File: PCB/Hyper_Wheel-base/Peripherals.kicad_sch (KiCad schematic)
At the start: 18 parts, among them J1-1 Conn_01x06_Socket, J1-2 Conn_01x06_Pin, J2-1 Conn_01x04_Socket, U13 AS5600L-ASOM, U14 DRV5032FCDBZR, U3 AS5600L-ASOM, U8 DRV5032FCDBZR

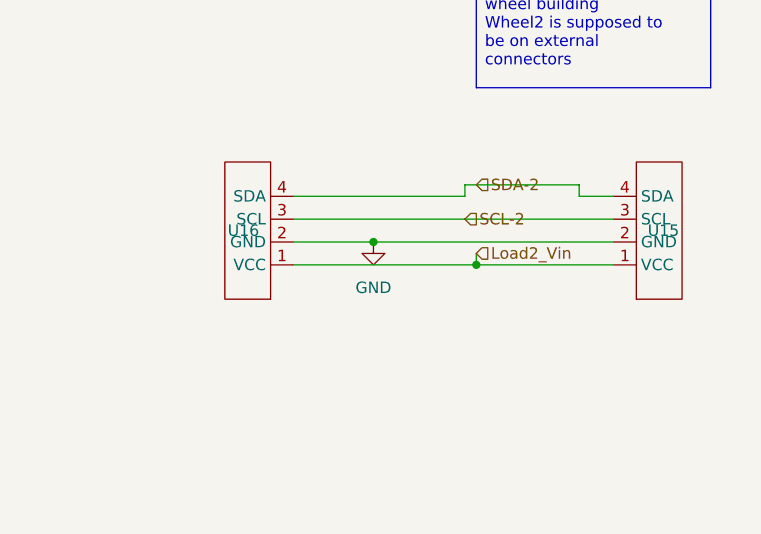
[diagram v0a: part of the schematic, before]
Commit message: Rev B Xiao.  migrated changes to main
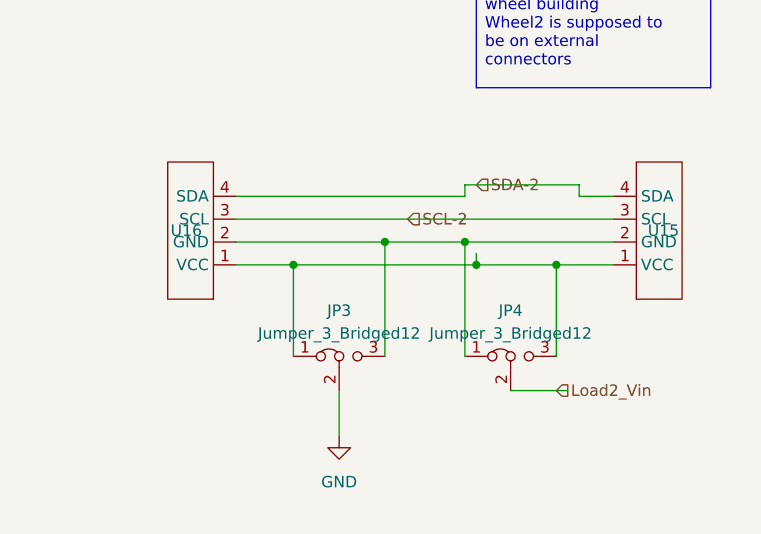
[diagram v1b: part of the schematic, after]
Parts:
- added JP3, JP4: Jumper_3_Bridged12, Jumper:SolderJumper-3_P1.3mm_Bridged12_Pad1.0x1.5mm, symbol Jumper:Jumper_3_Bridged12
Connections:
- net GND: now also JP3.2 (C); no longer U15.2 (GND), U16.2 (GND)
- net Load2_Vin: now also JP4.2 (C); no longer U15.1 (VCC), U16.1 (VCC)
- new net: JP3.1 (A), JP4.3 (B), U15.1 (VCC), U16.1 (VCC)
- new net: JP3.3 (B), JP4.1 (A), U15.2 (GND), U16.2 (GND)
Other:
- moved on the sheet: U16
